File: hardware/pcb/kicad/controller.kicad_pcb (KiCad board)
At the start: 6 copper layers, 160 x 130 mm, 29 parts, among them J1 48V_INPUT_10A, J10 ESTOP_RED_KEYED_DUAL_CHANNEL, J11 SAFETY_GATE_OUTPUT, J2 12V_OUTPUT_16A, J3 JETSON_DEVKIT_12V_5A, J4 JETSON_MCU_BACKPLANE, J5 CAN_A, J6 CAN_B, U1 LM5069_HOTSWAP, U2 DCM3623_48V_12V_240W, U3 JETSON_12V_EFUSE_5A, U4 BUCK_12V_3V3_5A, U5 CH32V307_CARRIER, U6 ISO1042DW, U7 3V3_5V_ISOLATED_DC_DC, U8 DUAL_CHANNEL_SAFETY_GATE_CARR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

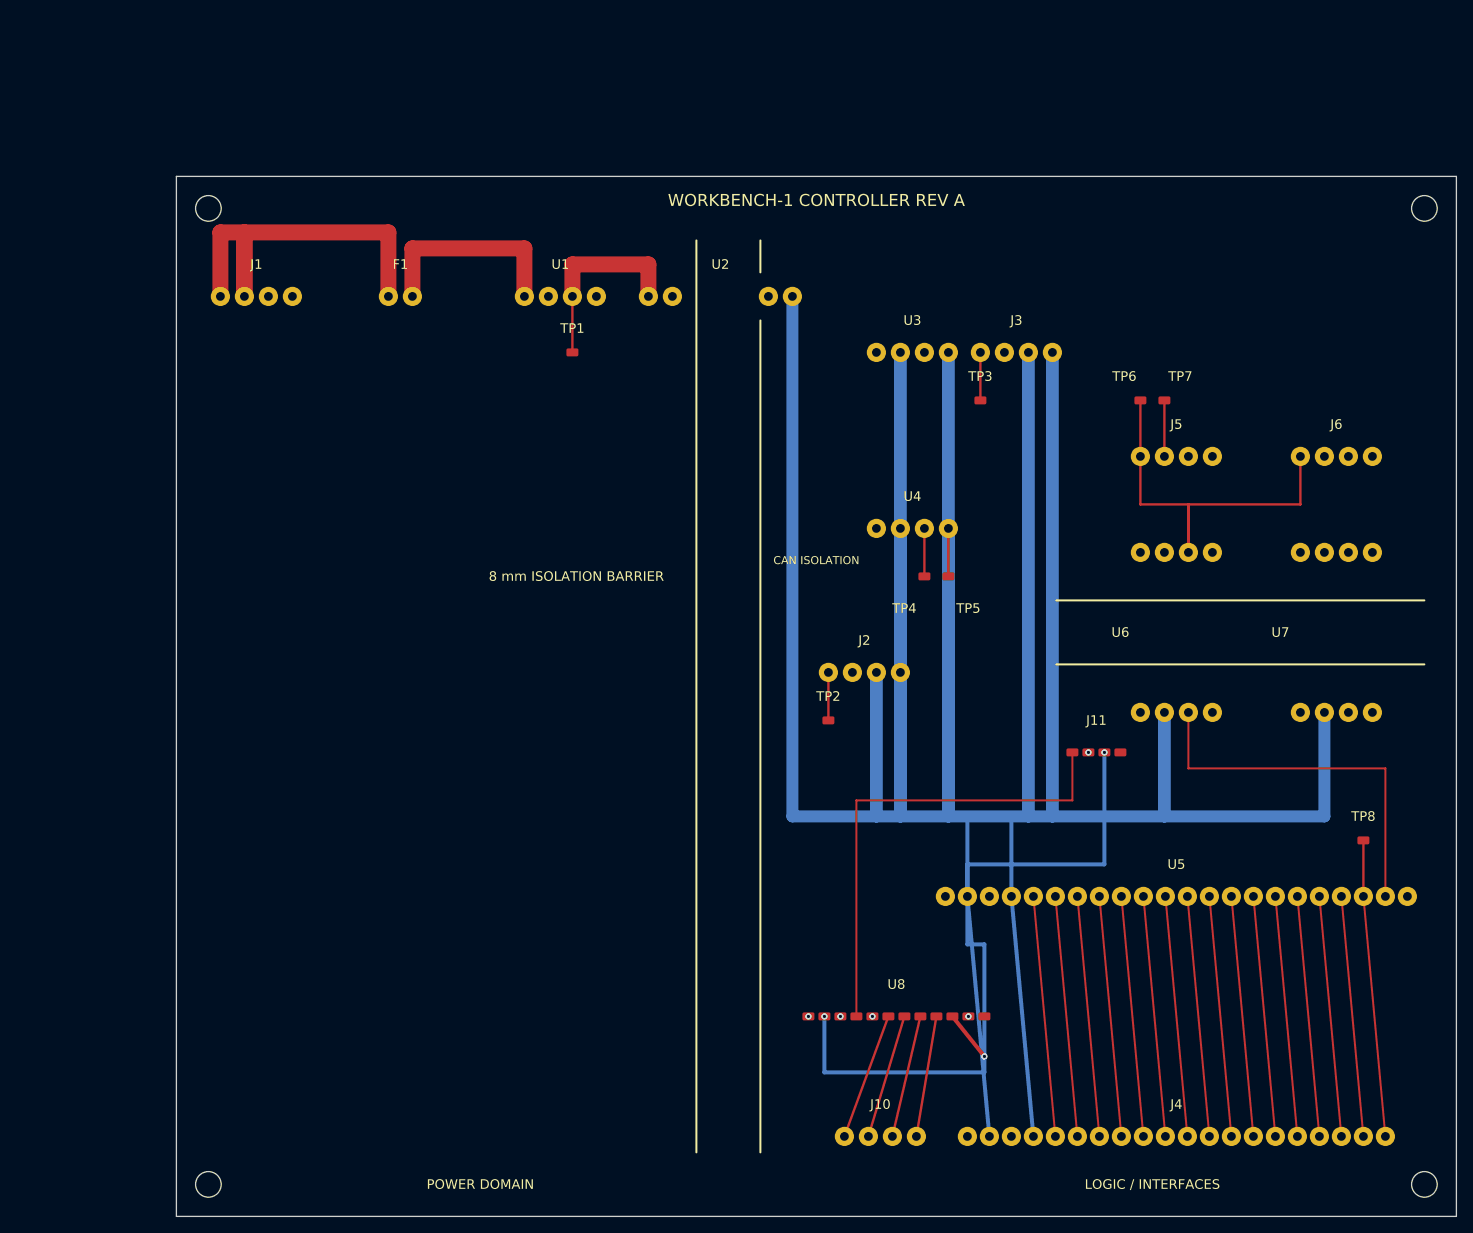
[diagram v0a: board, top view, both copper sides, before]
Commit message: feat(hardware): complete service robot engineering baseline
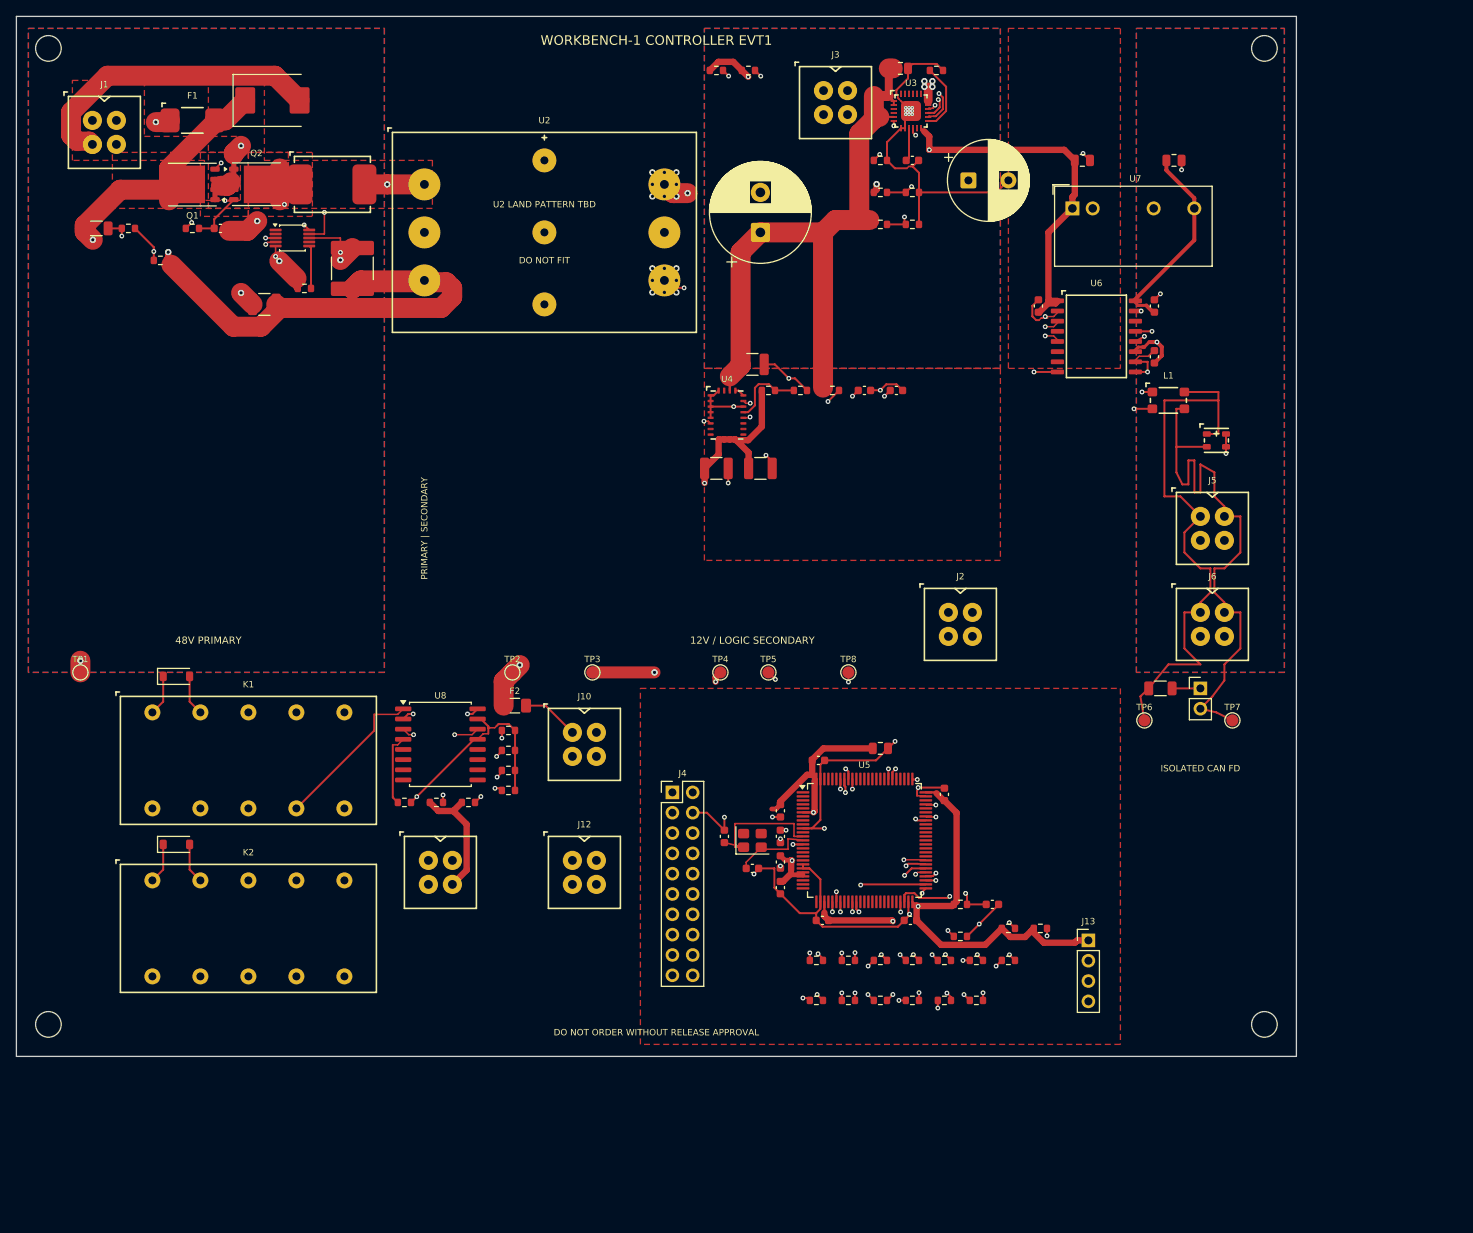
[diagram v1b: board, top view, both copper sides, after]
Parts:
- added C1: 1uF 100V, C_1210_3225Metric, F.Cu at (31.0, 36.0)
- added C10: 100nF, C_0603_1608Metric, F.Cu at (95.5, 102.5)
- added C11: 100nF, C_0603_1608Metric, F.Cu at (95.5, 105.7)
- added C12: 100nF, C_0603_1608Metric, F.Cu at (95.5, 108.9)
- added C13: 100nF, C_0603_1608Metric, F.Cu at (100.8, 113.0)
- added C14: 100nF, C_0603_1608Metric, F.Cu at (111.8, 113.0)
- added C15: 100nF, C_0603_1608Metric, F.Cu at (116.0, 97.2)
- added C16: 100nF, C_0603_1608Metric, F.Cu at (100.2, 93.0)
- added C17: 4.7uF, C_0805_2012Metric, F.Cu at (108.0, 91.5)
- added C18: 100nF, C_0603_1608Metric, F.Cu at (112.0, 18.0)
- added C19: 100nF, C_0603_1608Metric, F.Cu at (122.0, 111.0)
- added C2: 10uF 100V, C_2220_5750Metric, F.Cu at (42.0, 31.5)
- added C20: 1uF 10V, C_0603_1608Metric, F.Cu at (110.0, 46.8)
- added C3: 470uF 25V, CP_Radial_D12.5mm_P5.00mm, F.Cu at (93.0, 27.0)
- added C4: 1uF 25V, C_0805_2012Metric, F.Cu at (110.5, 6.50)
- added C40: 100nF, C_0603_1608Metric, F.Cu at (127.8, 36.2)
- added C41: 100nF, C_0603_1608Metric, F.Cu at (142.2, 36.2)
- added C42: 4.7uF, C_0805_2012Metric, F.Cu at (133.2, 18.0)
- added C43: 4.7uF, C_0805_2012Metric, F.Cu at (144.7, 18.0)
- added C44: 100nF, C_0603_1608Metric, F.Cu at (142.2, 42.5)
- added C5: 220uF 25V, CP_Radial_D10.0mm_P5.00mm, F.Cu at (119.0, 20.5)
- added C6: 22uF 25V, C_1210_3225Metric, F.Cu at (92.0, 43.5)
- added C7: 47uF 10V, C_1210_3225Metric, F.Cu at (87.5, 56.5)
- added C8: 47uF 10V, C_1210_3225Metric, F.Cu at (93.0, 56.5)
- added C9: 100nF, C_0603_1608Metric, F.Cu at (95.5, 99.3)
- added CG1: 4.7nF 100V, C_0603_1608Metric, F.Cu at (25.5, 26.5)
- added CSS4: 22nF, C_0603_1608Metric, F.Cu at (106.0, 46.8)
- added CY1: 18pF, C_0603_1608Metric, F.Cu at (88.5, 102.5)
- added CY2: 18pF, C_0603_1608Metric, F.Cu at (92.0, 106.5)
- added D1: SMCJ58A, D_SMC, F.Cu at (32.0, 10.5)
- added D2: CAN FD TVS, CAN_TVS, F.Cu at (150.0, 53.0)
- added D3: FLYBACK, D_SOD-123, F.Cu at (20.0, 82.5)
- added D4: FLYBACK, D_SOD-123, F.Cu at (20.0, 103.5)
- added F2: PTC 0.25A, Fuse_1206_3216Metric, F.Cu at (62.3, 86.2)
- added J12: DUAL MANUAL RESET, MicroFit_2x2, F.Cu at (71.0, 107.0)
- added J13: WCH DEBUG, PinHeader_1x04_P2.54mm_Vertical, F.Cu at (134.0, 115.5)
- added JP1: CAN TERM, PinHeader_1x02_P2.54mm_Vertical, F.Cu at (148.0, 84.0)
- added K1: FORCE-GUIDED 12V A, Panasonic_SFM4, F.Cu at (29.0, 93.0)
- added K2: FORCE-GUIDED 12V B, Panasonic_SFM4, F.Cu at (29.0, 114.0)
- added L1: 100R@100MHz, ACT45B, F.Cu at (144.0, 48.0)
- added Q1: 150V N-MOS, Infineon_PG-TDSON-8_6.15x5.15mm, F.Cu at (22.0, 21.0)
- added Q2: 150V N-MOS, Infineon_PG-TDSON-8_6.15x5.15mm, F.Cu at (30.0, 21.0)
- added R30: 33R, R_0603_1608Metric, F.Cu at (100.0, 118.0)
- added R31: 33R, R_0603_1608Metric, F.Cu at (104.0, 118.0)
- added R32: 33R, R_0603_1608Metric, F.Cu at (108.0, 118.0)
- added R33: 33R, R_0603_1608Metric, F.Cu at (112.0, 118.0)
- added R34: 33R, R_0603_1608Metric, F.Cu at (116.0, 118.0)
- added R35: 33R, R_0603_1608Metric, F.Cu at (120.0, 118.0)
- added R36: 33R, R_0603_1608Metric, F.Cu at (124.0, 118.0)
- added R37: 33R, R_0603_1608Metric, F.Cu at (100.0, 123.0)
- added R38: 33R, R_0603_1608Metric, F.Cu at (104.0, 123.0)
- added R39: 33R, R_0603_1608Metric, F.Cu at (108.0, 123.0)
- added R40: 33R, R_0603_1608Metric, F.Cu at (112.0, 123.0)
- added R41: 33R, R_0603_1608Metric, F.Cu at (116.0, 123.0)
- added R42: 33R, R_0603_1608Metric, F.Cu at (120.0, 123.0)
- added R43: 100k, R_0603_1608Metric, F.Cu at (118.0, 115.0)
- added R44: 100k, R_0603_1608Metric, F.Cu at (61.5, 91.8)
- added R45: 100k, R_0603_1608Metric, F.Cu at (61.5, 94.3)
- added R46: 100k, R_0603_1608Metric, F.Cu at (102.0, 46.8)
- added R47: 10k, R_0603_1608Metric, F.Cu at (91.5, 6.75)
- added R48: 3.00k 1%, R_0603_1608Metric, F.Cu at (108.0, 18.0)
- added R49: 10k, R_0603_1608Metric, F.Cu at (52.5, 98.3)
- added R50: 10k, R_0603_1608Metric, F.Cu at (56.5, 98.3)
- added R51: 10k, R_0603_1608Metric, F.Cu at (115.0, 6.75)
- added R52: 4.7k, R_0603_1608Metric, F.Cu at (61.5, 96.8)
- added R53: 4.7k, R_0603_1608Metric, F.Cu at (48.5, 98.3)
- added R54: 10k, R_0603_1608Metric, F.Cu at (118.0, 111.0)
- added R55: 4.7k, R_0603_1608Metric, F.Cu at (124.0, 114.0)
- added R56: 4.7k, R_0603_1608Metric, F.Cu at (128.0, 114.0)
- added R57: 100k, R_0603_1608Metric, F.Cu at (61.5, 89.3)
- added R58: 120R 1%, R_1206_3216Metric, F.Cu at (143.0, 84.0)
- added R59: 73.2k 1%, R_0603_1608Metric, F.Cu at (108.0, 26.0)
- added R60: 10.0k 1%, R_0603_1608Metric, F.Cu at (112.0, 26.0)
- added RFB1: 45.0k 1%, R_0603_1608Metric, F.Cu at (94.0, 46.8)
- added RFB2: 10.0k 1%, R_0603_1608Metric, F.Cu at (98.0, 46.8)
- added RG1: 22k, R_0603_1608Metric, F.Cu at (22.0, 26.5)
- added RPG1: 453k 1%, R_0603_1608Metric, F.Cu at (108.0, 22.0)
- added RPG2: 56.0k 1%, R_0603_1608Metric, F.Cu at (112.0, 22.0)
- added RPG3: 10k, R_0603_1608Metric, F.Cu at (87.5, 6.75)
- added RS1: 6mR 3W 1%, Sense_3637, F.Cu at (39.5, 21.0)
- added RSH1: 510k, R_0603_1608Metric, F.Cu at (36.0, 34.0)
- added RUV1: 19.6M 1%, R_1206_3216Metric, F.Cu at (10.0, 26.5)
- added RUV2: 133k 1%, R_0603_1608Metric, F.Cu at (14.0, 26.5)
- added RUV3: 162k 1%, R_0603_1608Metric, F.Cu at (18.0, 30.5)
- added Y1: 8MHz, Crystal_SMD_3225-4Pin_3.2x2.5mm, F.Cu at (92.0, 103.0)
- F1: value FUSE_10A -> 10A 125V; footprint (none) -> Fuse_4510
- J1: value 48V_INPUT_10A -> 48V INPUT; footprint (none) -> MicroFit_2x2
- J10: value ESTOP_RED_KEYED_DUAL_CHANNEL -> DUAL ESTOP LOOP; footprint (none) -> MicroFit_2x2
- J11: value SAFETY_GATE_OUTPUT -> SAFETY OUTPUT; footprint (none) -> MicroFit_2x2
- J2: value 12V_OUTPUT_16A -> 12V MOTOR AUX; footprint (none) -> MicroFit_2x2
- J3: value JETSON_DEVKIT_12V_5A -> JETSON DEVKIT 12V; footprint (none) -> MicroFit_2x2
- J4: value JETSON_MCU_BACKPLANE -> JETSON MCU BACKPLANE; footprint (none) -> PinHeader_2x10_P2.54mm_Vertical
- J5: value CAN_A -> CAN A; footprint (none) -> MicroFit_2x2
- J6: value CAN_B -> CAN B; footprint (none) -> MicroFit_2x2
- TP1, TP2, TP3, TP4, TP5, TP6, TP7, TP8: footprint (none) -> TestPoint_Pad_D1.5mm
- U1: value LM5069_HOTSWAP -> LTC4368HMS-2; footprint (none) -> MSOP-10_3x3mm_P0.5mm
- U2: value DCM3623_48V_12V_240W -> ISOLATED 48V-12V 240W (TBD); footprint (none) -> Isolated_48V_12V_240W_TBD
- U3: value JETSON_12V_EFUSE_5A -> TPS26633RGE; footprint (none) -> TPS26633_RGE24
- U4: value BUCK_12V_3V3_5A -> RPL-5.0 3V3/5A; footprint (none) -> RPL-5.0_QFN24
- U5: value CH32V307_CARRIER -> CH32V307VCT6; footprint (none) -> LQFP-100_14x14mm_P0.5mm
- U6: footprint (none) -> ISO1042_DW16_HV
- U7: value 3V3_5V_ISOLATED_DC_DC -> 3V3-5V ISO 1W; footprint (none) -> Converter_DCDC_muRata_MEJ1SxxxxSC_THT
- U8: value DUAL_CHANNEL_SAFETY_GATE_CARRIER -> ESTOP DIAGNOSTIC OPTO; footprint (none) -> SOIC-16W_7.5x10.3mm_P1.27mm
- moved J11 83.4 mm to (53.0, 107.0)
- moved J4 76.3 mm to (82.0, 97.0)
- moved TP1 73.4 mm to (8.00, 82.0)
- moved TP8 67.7 mm to (104.0, 82.0)
- moved U8 66.4 mm to (53.0, 91.0)
- moved U7 62.4 mm to (132.0, 24.0)
- moved J10 61.4 mm to (71.0, 91.0)
- moved TP3 59.2 mm to (72.0, 82.0)
- moved TP7 40.9 mm to (152.0, 88.0)
- moved TP6 40.0 mm to (141.0, 88.0)
- moved TP2 40.0 mm to (62.0, 82.0)
- moved U5 39.6 mm to (106.0, 103.0)
- moved J3 38.6 mm to (102.4, 10.8)
- moved U6 38.3 mm to (135.0, 40.0)
- moved U1 34.3 mm to (34.5, 27.7)
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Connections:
- J10 pad 1: ESTOP_CH_A_OUT -> ESTOP_12V
- J10 pad 3: ESTOP_CH_B_OUT -> ESTOP_12V
- J11 pad 4: (no net) -> 3V3_LOGIC
- J4 pad 8: MOTOR_ENABLE_REQ -> JETSON_ENABLE_REQ
- U1 pad 1: VBAT_FUSED -> GND_PWR
- U1 pad 3: VBAT_PROTECTED -> OV_SET
- U1 pad 4: GND_PWR -> UV_SET
- U2 pad 3: 12V_ISO -> (no net)
- U2 pad 4: GND -> 12V_ISO
- U3 pad 2: GND -> 12V_ISO
- U3 pad 3: JETSON_12V -> (no net)
- U3 pad 4: GND -> (no net)
- U4 pad 1: 12V_ISO -> GND
- U4 pad 3: 3V3_LOGIC -> GND
- U5 pad 1: 3V3_LOGIC -> (no net)
- U5 pad 10: MOTOR_CS1 -> GND
- U5 pad 11: MOTOR_CS2 -> 3V3_LOGIC
- U5 pad 12: MOTOR_CS3 -> OSC_IN
- U5 pad 13: MOTOR_CS4 -> OSC_OUT
- U5 pad 14: MOTOR_CS5 -> MCU_RESET
- U5 pad 15: I2C_SDA -> (no net)
- U5 pad 16: I2C_SCL -> (no net)
- U5 pad 17: ESTOP_SENSE -> (no net)
- U5 pad 18: UART_TX -> (no net)
- U5 pad 19: UART_RX -> GND
- U5 pad 2: GND -> (no net)
- U5 pad 20: MCU_RESET -> GND
- U5 pad 21: CAN_TX -> 3V3_LOGIC
- U5 pad 22: CAN_RX -> 3V3_LOGIC
- U5 pad 3: 3V3_LOGIC -> (no net)
- U5 pad 4: GND -> (no net)
- U5 pad 5: SPI_SCLK -> (no net)
- U5 pad 6: SPI_MOSI -> 3V3_LOGIC
- U5 pad 7: SPI_MISO -> (no net)
- U5 pad 8: MOTOR_ENABLE_REQ -> (no net)
- U5 pad 9: MOTOR_CS0 -> (no net)
- U6 pad 1: 5V_CAN_ISO -> 3V3_LOGIC
- U6 pad 2: GND_CAN_ISO -> GND
- U6 pad 3: CANH -> CAN_TX
- U6 pad 4: CANL -> (no net)
- U6 pad 5: 3V3_LOGIC -> CAN_RX
- U6 pad 6: GND -> (no net)
- U6 pad 7: CAN_TX -> (no net)
- U6 pad 8: CAN_RX -> GND
- U7 pad 1: 5V_CAN_ISO -> 3V3_LOGIC
- U7 pad 2: GND_CAN_ISO -> GND
- U7 pad 5: 3V3_LOGIC -> GND_CAN_ISO
- U7 pad 7: (no net) -> 5V_CAN_ISO
- U8 pad 1: 12V_ISO -> ESTOP_CH_A_RETURN
- U8 pad 10: GND -> (no net)
- U8 pad 11: 3V3_LOGIC -> (no net)
- U8 pad 2: GND -> U8_LED_A_K
- U8 pad 3: MOTOR_ENABLE_REQ -> ESTOP_CH_B_RETURN
- U8 pad 4: MOTOR_ENABLE_SAFE -> U8_LED_B_K
- U8 pad 5: ESTOP_SENSE -> (no net)
- U8 pad 6: ESTOP_CH_A_OUT -> (no net)
- U8 pad 7: ESTOP_CH_A_RETURN -> (no net)
- U8 pad 8: ESTOP_CH_B_OUT -> (no net)
- U8 pad 9: ESTOP_CH_B_RETURN -> (no net)
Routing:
- net GND: track 1029.4 -> 582.5 mm, vias 3 -> 38
- net 3V3_LOGIC: track 213.9 -> 487.8 mm, vias 1 -> 9
- net RELAY_B_NC: track 0.00 -> 113.5 mm, vias 0 -> 2
- net RELAY_A_NC: track 0.00 -> 107.3 mm, vias 0 -> 2
- net JETSON_12V: track 36.0 -> 141.9 mm, vias 0 -> 6
- net ESTOP_A_MON: track 0.00 -> 78.0 mm, vias 0 -> 3
- net VBAT_PROTECTED: track 24.5 -> 100.1 mm, vias 0 -> 5
- net ESTOP_B_MON: track 0.00 -> 72.2 mm, vias 0 -> 3
- net RESET_CH_B_RETURN: track 0.00 -> 70.3 mm
- net RESET_CH_A_RETURN: track 0.00 -> 68.2 mm
- net ESTOP_CH_B_RETURN: track 15.2 -> 79.1 mm, vias 0 -> 1
- net ESTOP_CH_A_RETURN: track 15.7 -> 74.1 mm
- net ESTOP_SENSE: track 170.3 -> 113.0 mm
- net VBAT_RAW: track 53.0 -> 9.88 mm, vias 0 -> 1
- net MOTOR_ENABLE_SAFE: track 60.0 -> 17.5 mm
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- added copper zone on In2.Cu, net 12V_ISO
- added copper zone on F.Cu, net 3V3_LOGIC
- added copper zone on In5.Cu, net 3V3_LOGIC
- added copper zone on In5.Cu, net 5V_CAN_ISO
- added copper zone on F.Cu, net FET_COMMON
- added copper zone on In1.Cu, net GND
- added copper zone on In4.Cu, net GND
- added copper zone on B.Cu, net GND_CAN_ISO
- added copper zone on F.Cu, net GND_CAN_ISO
- added copper zone on In1.Cu, net GND_CAN_ISO
- added copper zone on In4.Cu, net GND_CAN_ISO
- added copper zone on B.Cu, net GND_PWR
- added copper zone on F.Cu, net GND_PWR
- added copper zone on In1.Cu, net GND_PWR
- added copper zone on F.Cu, net INPUT_SENSE
- added copper zone on B.Cu, net JETSON_12V
- added copper zone on F.Cu, net JETSON_12V
- added copper zone on In3.Cu, net JETSON_12V
- added copper zone on F.Cu, net VBAT_FUSED
- added copper zone on F.Cu, net VBAT_PROTECTED
- added copper zone on F.Cu, net VBAT_RAW
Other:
- copper layers 6 -> 8
- board text added: "12V / LOGIC SECONDARY"
- board text added: "48V PRIMARY"
- board text added: "DO NOT FIT"
- board text added: "DO NOT ORDER WITHOUT RELEASE APPROVAL"
- board text added: "FAB: ENIG | THK 1.60 +/- 0.16 MM (MASK EXCL)"
- board text added: "FAB: U3 HDI 9x 0.45/0.15 FILL/CAP/PLANARIZE"
- board text added: "ISOLATED CAN FD"
- board text added: "PRIMARY | SECONDARY"
- board text added: "U2 LAND PATTERN TBD"
- board text added: "WORKBENCH-1 CONTROLLER EVT1"
- board text removed: "8 mm ISOLATION BARRIER"
- board text removed: "CAN ISOLATION"
- board text removed: "LOGIC / INTERFACES"
- board text removed: "POWER DOMAIN"
- board text removed: "WORKBENCH-1 CONTROLLER REV A"
